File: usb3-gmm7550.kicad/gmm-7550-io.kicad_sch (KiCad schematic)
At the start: 17 parts, among them J4 10144517-061802LF, SW2 SW_Push, SW3 SW_Push

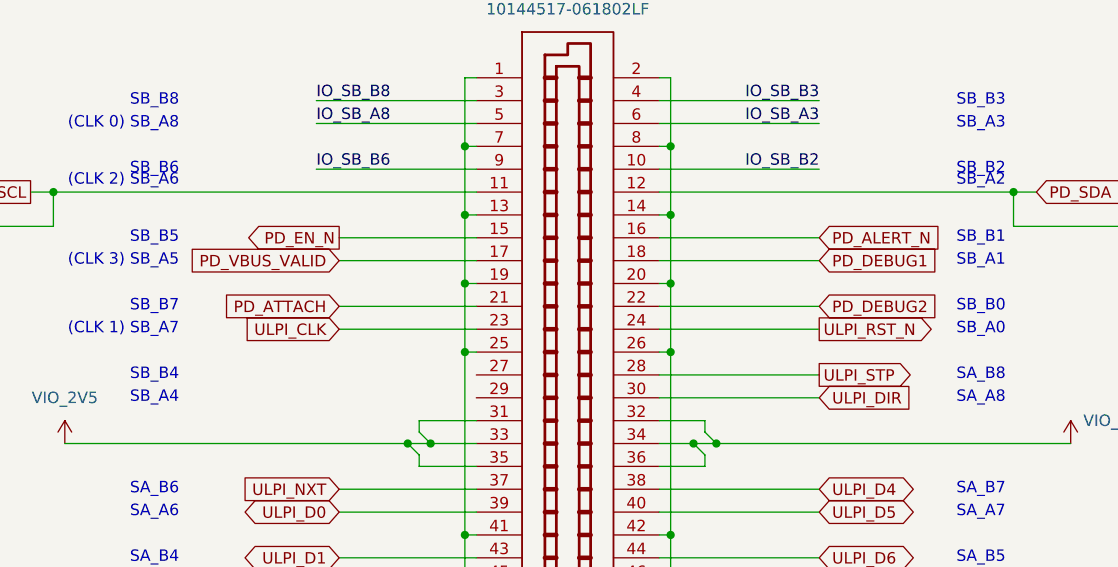
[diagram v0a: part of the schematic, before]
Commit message: Layout WIP: split power plane (internal layer 2)
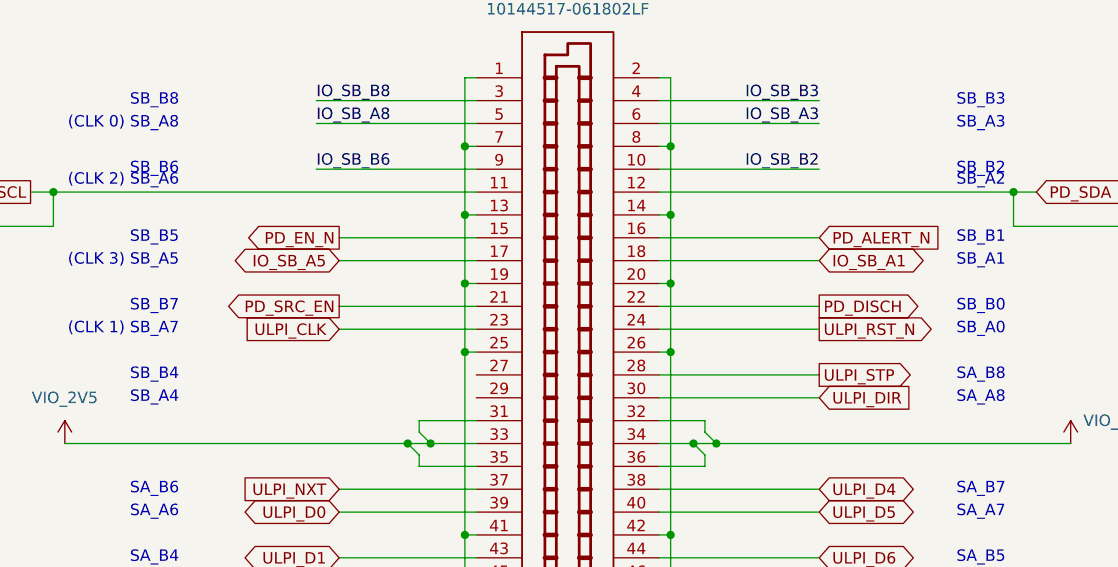
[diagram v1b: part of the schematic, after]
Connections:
- net PD_ATTACH renamed PD_SRC_EN
- net PD_DEBUG1 renamed IO_SB_A1
- net PD_DEBUG2 renamed PD_DISCH
- net PD_VBUS_VALID renamed IO_SB_A5
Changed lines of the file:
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@@
-		)
-	)
-	(global_label "PD_VBUS_VALID"
-		(shape input)
-		(at 119.38 53.34 180)
-		(fields_autoplaced yes)
-		(effects
-			(font
-				(size 1.27 1.27)
-			)
-			(justify right)
-		)
-		(property "Intersheetrefs" "${INTERSHEET_REFS}"
-			(at 101.9409 53.34 0)
-			(effects
-				(font
-					(size 1.27 1.27)
-				)
-				(justify right)
-				(hide yes)
-			)
 		)
 	)
@@
 		)
 	)
-	(global_label "PD_ATTACH"
-		(shape input)
-		(at 119.38 58.42 180)
-		(fields_autoplaced yes)
-		(effects
-			(font
-				(size 1.27 1.27)
-			)
-			(justify right)
-		)
-		(property "Intersheetrefs" "${INTERSHEET_REFS}"
-			(at 106.1743 58.42 0)
-			(effects
-				(font
-					(size 1.27 1.27)
-				)
-				(justify right)
-				(hide yes)
-			)
-		)
-	)
 	(global_label "ULPI_RST_N"
 		(shape output)
@@
 		(property "Intersheetrefs" "${INTERSHEET_REFS}"
 			(at 230.3716 49.53 0)
-			(effects
-				(font
-					(size 1.27 1.27)
-				)
-				(justify left)
-				(hide yes)
-			)
-		)
-	)
-	(global_label "PD_DEBUG2"
-		(shape input)
-		(at 172.72 58.42 0)
-		(fields_autoplaced yes)
-		(effects
-			(font
-				(size 1.27 1.27)
-			)
-			(justify left)
-		)
-		(property "Intersheetrefs" "${INTERSHEET_REFS}"
-			(at 186.7118 58.42 0)
 			(effects
 				(font
@@
 		)
 	)
+	(global_label "PD_SRC_EN"
+		(shape output)
+		(at 119.38 58.42 180)
+		(fields_autoplaced yes)
+		(effects
+			(font
+				(size 1.27 1.27)
+			)
+			(justify right)
+		)
+		(property "Intersheetrefs" "${INTERSHEET_REFS}"
+			(at 105.6906 58.42 0)
+			(effects
+				(font
+					(size 1.27 1.27)
+				)
+				(justify right)
+				(hide yes)
+			)
+		)
+	)
 	(global_label "USB1_CON"
 		(shape output)
@@
 		)
 	)
+	(global_label "PD_DISCH"
+		(shape output)
+		(at 172.72 58.42 0)
+		(fields_autoplaced yes)
+		(effects
+			(font
+				(size 1.27 1.27)
+			)
+			(justify left)
+		)
+		(property "Intersheetrefs" "${INTERSHEET_REFS}"
+			(at 184.8976 58.42 0)
+			(effects
+				(font
+					(size 1.27 1.27)
+				)
+				(justify left)
+				(hide yes)
+			)
+		)
+	)
 	(global_label "USB1_BUSDET"
 		(shape input)
@@
 		)
 	)
+	(global_label "IO_SB_A5"
+		(shape bidirectional)
+		(at 119.38 53.34 180)
+		(fields_autoplaced yes)
+		(effects
+			(font
+				(size 1.27 1.27)
+			)
+			(justify right)
+		)
+		(property "Intersheetrefs" "${INTERSHEET_REFS}"
+			(at 106.6354 53.34 0)
+			(effects
+				(font
+					(size 1.27 1.27)
+				)
+				(justify right)
+				(hide yes)
+			)
+		)
+	)
 	(global_label "PD_ALERT_N"
 		(shape input)
@@
 		)
 	)
-	(global_label "PD_DEBUG1"
-		(shape input)
+	(global_label "IO_SB_A1"
+		(shape bidirectional)
 		(at 172.72 53.34 0)
 		(fields_autoplaced yes)
@@
 		)
 		(property "Intersheetrefs" "${INTERSHEET_REFS}"
-			(at 186.7118 53.34 0)
-			(effects
-				(font
+			(at 185.4646 53.34 0)
+			(effects
+				(font
